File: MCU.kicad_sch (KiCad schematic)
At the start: 10 parts, among them P2 CONN_01X02, U1 STM32G0B1CBT, X3 TC2030-NL, Y1 830055299

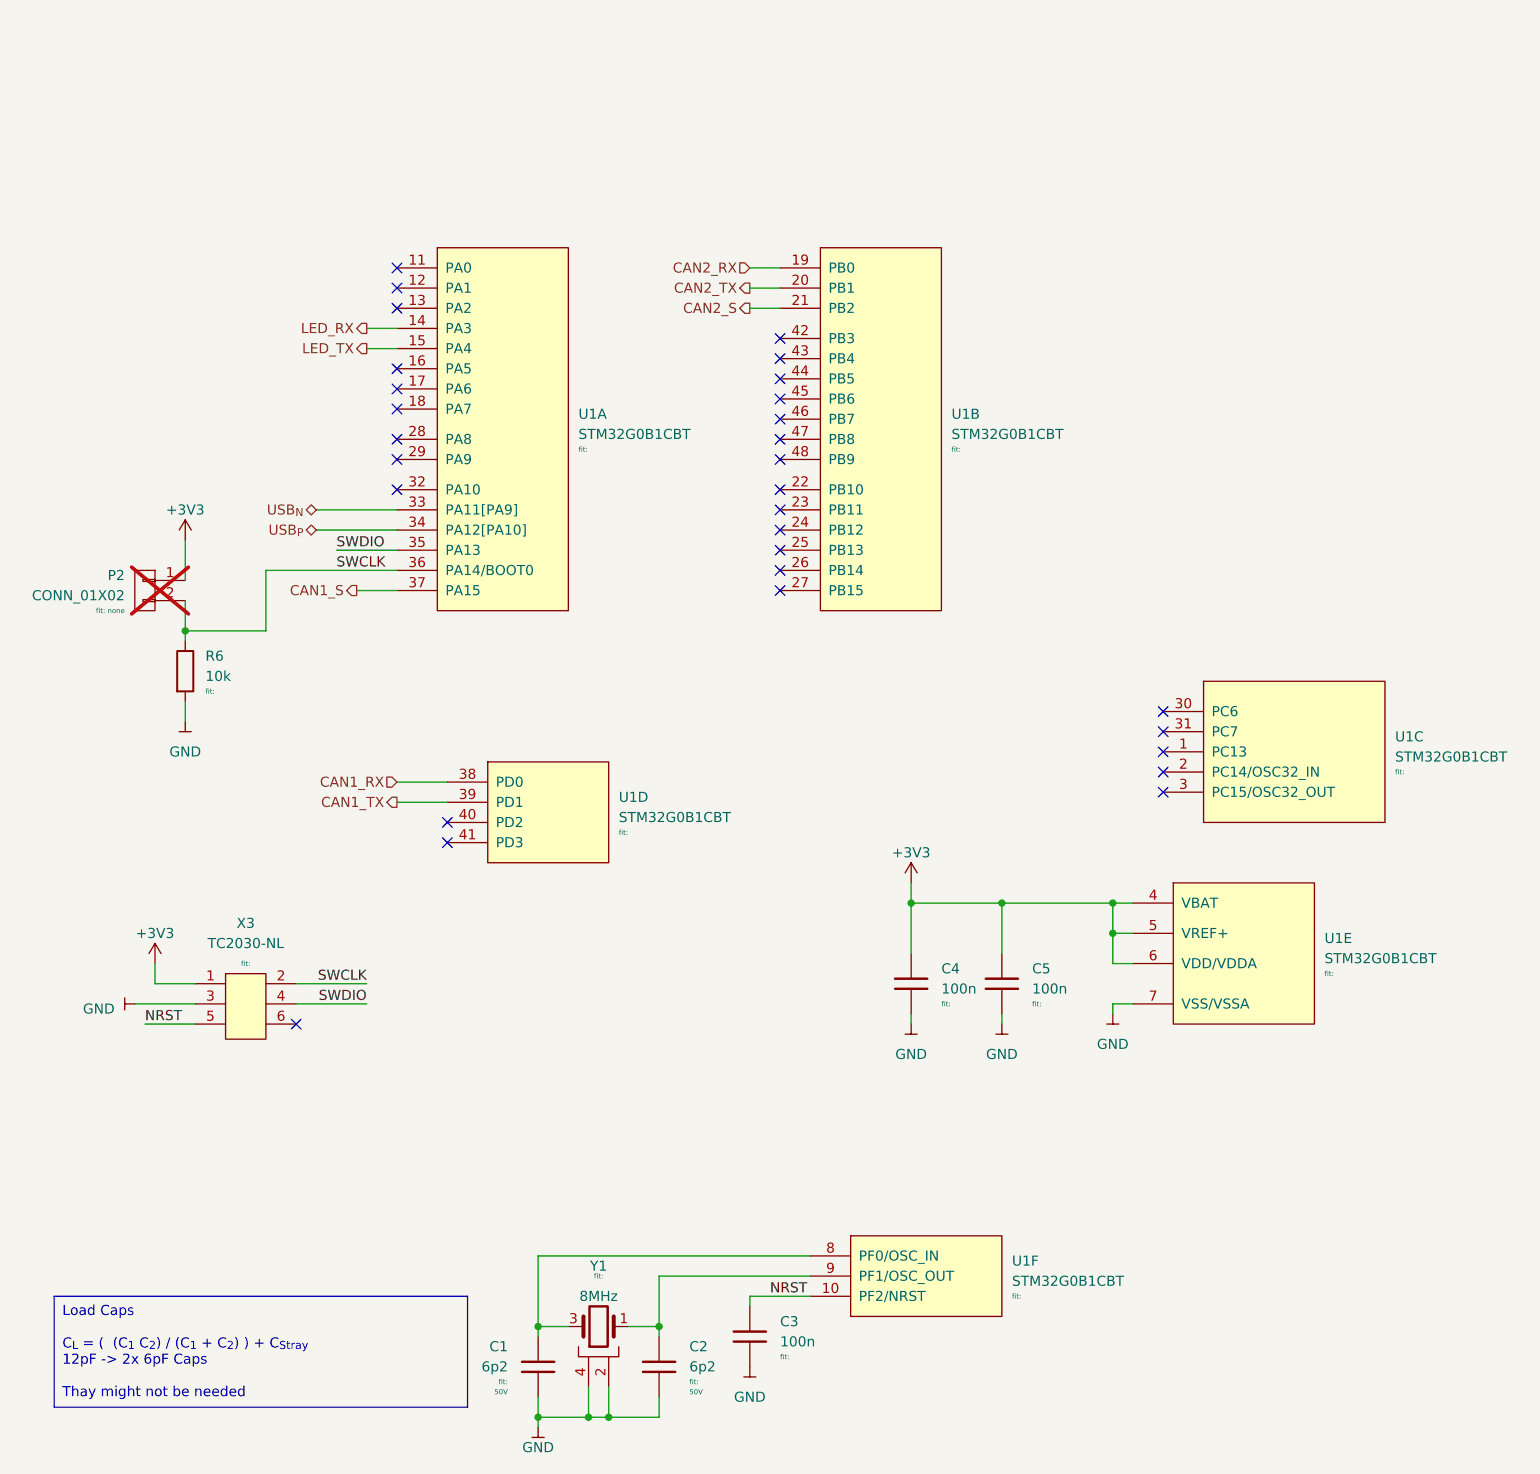
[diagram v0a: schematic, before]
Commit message: Save after recover
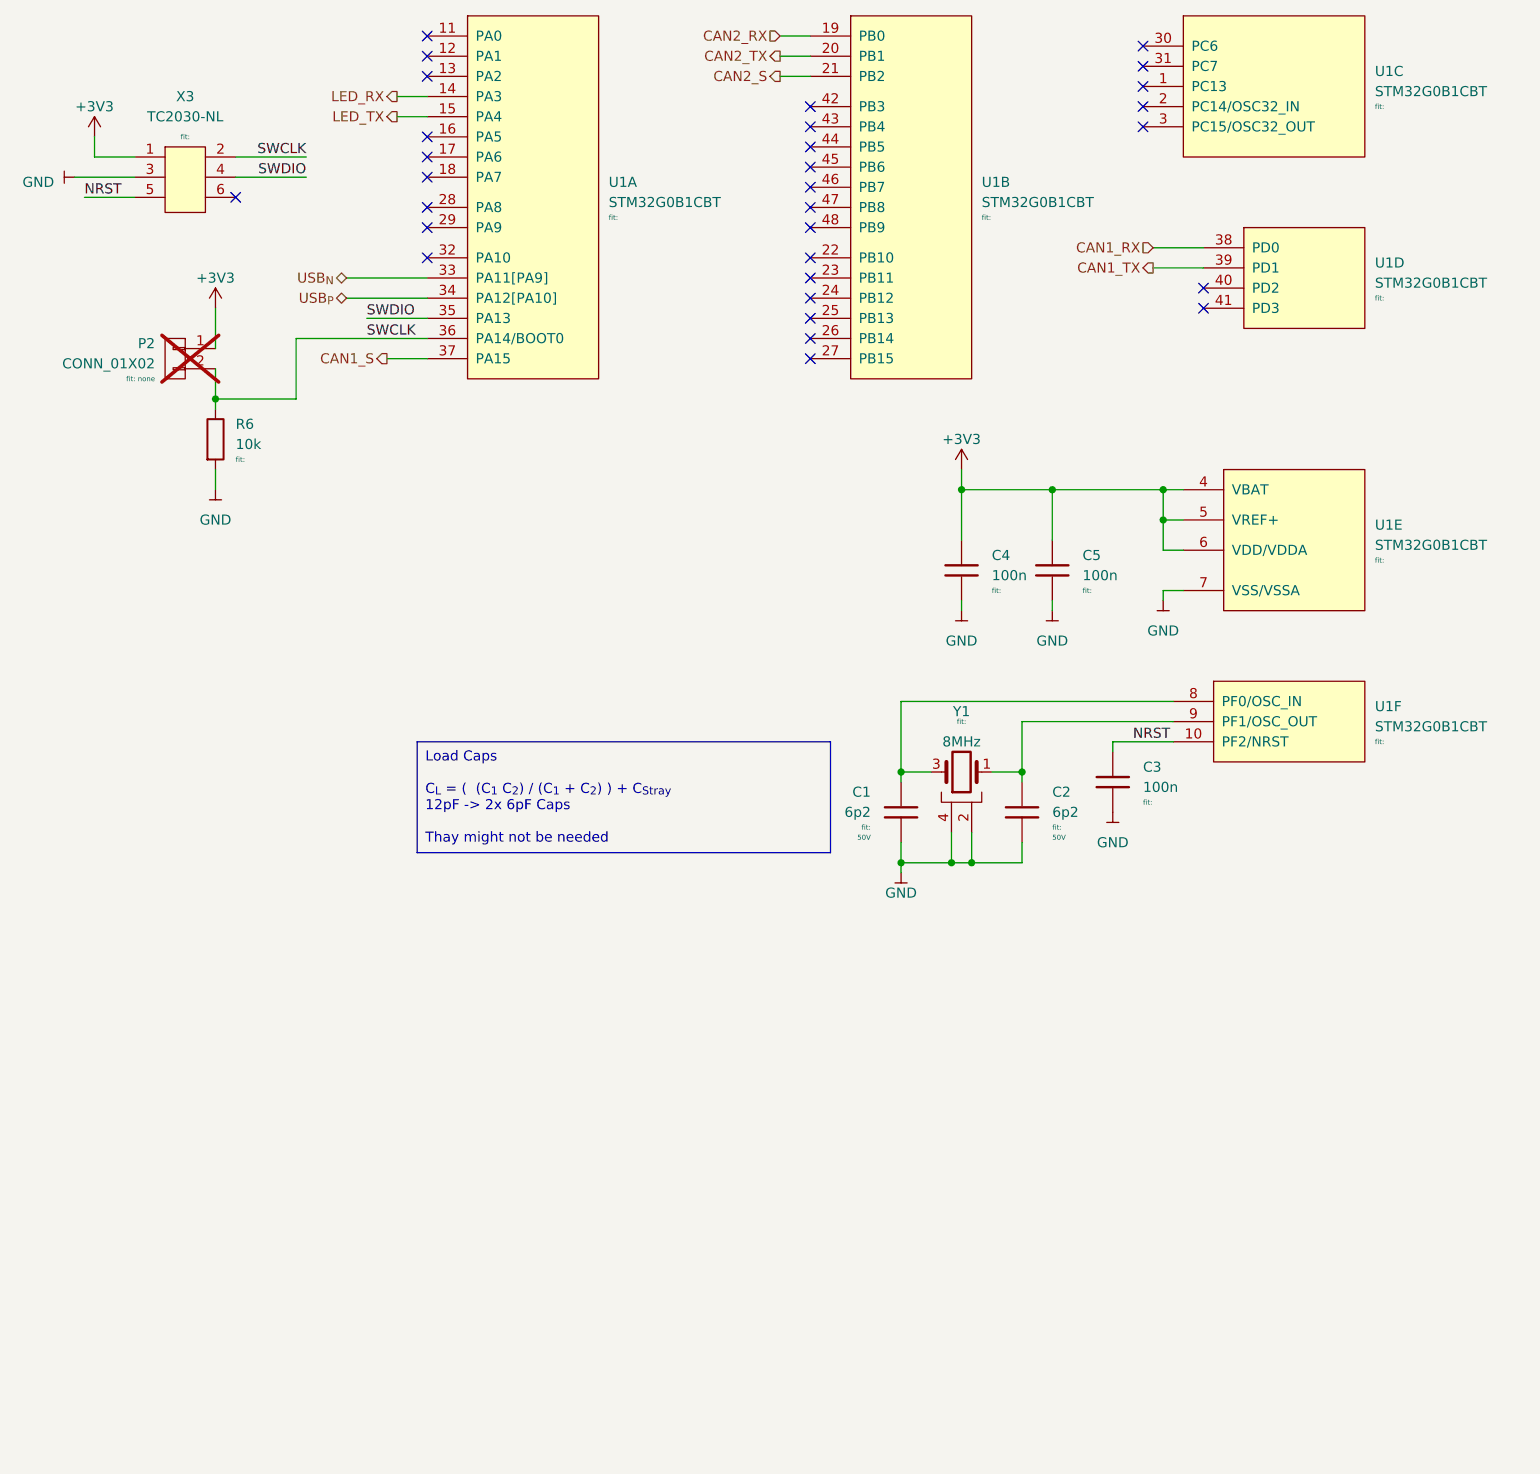
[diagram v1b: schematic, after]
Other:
- moved on the sheet: C1, C2, C3, C4, C5, P2, R6, U1A, U1B, U1C, U1D, U1E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
